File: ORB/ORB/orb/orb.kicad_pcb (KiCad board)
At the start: 2 copper layers, 132.1 x 82.5 mm, 6 parts, among them U1 Arduino_Nano, X1 14-Pin Plug, X2 14-Pin Plug, X3 14-Pin Plug, X4 14-Pin Plug

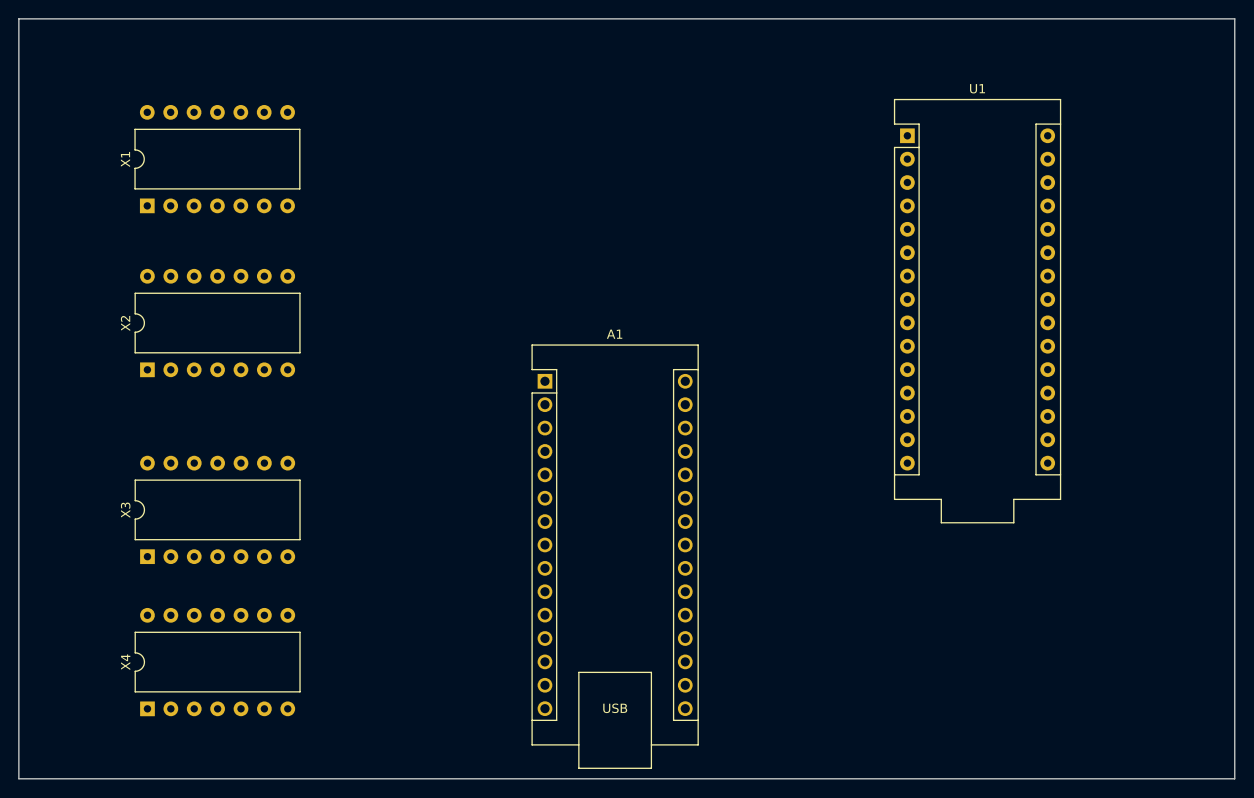
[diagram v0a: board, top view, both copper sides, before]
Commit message: Latest updates
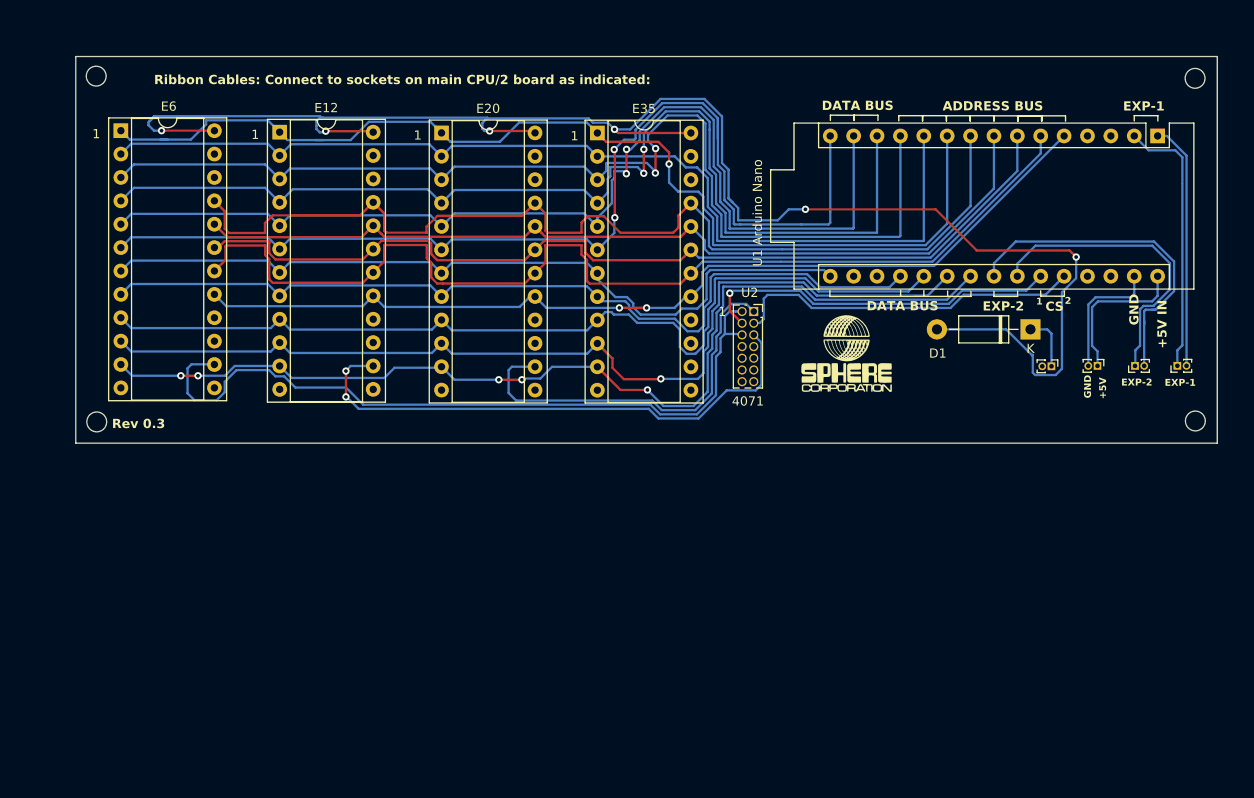
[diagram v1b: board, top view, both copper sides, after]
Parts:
- removed A1: Arduino_Nano_v3.x, Module:Arduino_Nano
- removed X1, X2, X3, X4: 14-Pin Plug, Package_DIP:DIP-14_W10.16mm
- added D1: 1N4001, Diode_THT:D_DO-41_SOD81_P10.16mm_Horizontal, F.Cu at (193.7, 75.6)
- added E12: MM1702A, Package_DIP:DIP-24_W10.16mm_Socket, F.Cu at (112.2, 54.2)
- added E20: MM1702A, Package_DIP:DIP-24_W10.16mm_Socket, F.Cu at (129.7, 54.3)
- added E35: MM1702A, Package_DIP:DIP-24_W10.16mm_Socket, F.Cu at (146.7, 54.3)
- added E6: MM1702A, Package_DIP:DIP-24_W10.16mm_Socket, F.Cu at (94.9, 54.1)
- added G***: LOGO, Arduino:sphere-corp-board-logo, F.Cu at (173.8, 78.2)
- added G***: LOGO, Arduino:orb-logo, B.Cu at (201.7, 61.2)
- added J1: Conn_01x02_Socket, Connector_PinHeader_1.00mm:PinHeader_1x02_P1.00mm_Vertical, F.Cu at (201.0, 79.6)
- added J2: Conn_01x02_Socket, Connector_PinHeader_1.00mm:PinHeader_1x02_P1.00mm_Vertical, F.Cu at (209.7, 79.6)
- added J3: Conn_01x02_Socket, Connector_PinHeader_1.00mm:PinHeader_1x02_P1.00mm_Vertical, F.Cu at (205.1, 79.6)
- added J4: Conn_01x02_Socket, Connector_PinHeader_1.00mm:PinHeader_1x02_P1.00mm_Vertical, F.Cu at (196.0, 79.7)
- added U3: 4071, Connector_PinSocket_1.27mm:PinSocket_2x07_P1.27mm_Vertical, F.Cu at (163.7, 73.7)
- moved U1 27.2 mm to (207.5, 54.6), turned to -90 degrees
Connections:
- U1 pad 1: unconnected-(U1-D1/TX-Pad1) -> Net-(J2-Pin_2)
- U1 pad 10: unconnected-(U1-D7-Pad10) -> Net-(E12-A2)
- U1 pad 11: unconnected-(U1-D8-Pad11) -> Net-(E12-A1)
- U1 pad 12: unconnected-(U1-~D9-Pad12) -> Net-(E12-A0)
- U1 pad 13: unconnected-(U1-~D10-Pad13) -> Net-(E12-D0)
- U1 pad 14: unconnected-(U1-~D11-Pad14) -> Net-(E12-D1)
- U1 pad 15: unconnected-(U1-D12-Pad15) -> Net-(E12-D2)
- U1 pad 16: unconnected-(U1-D13-Pad16) -> Net-(E12-D3)
- U1 pad 19: unconnected-(U1-A0/D14-Pad19) -> Net-(E12-D4)
- U1 pad 2: unconnected-(U1-D0/RX-Pad2) -> Net-(J2-Pin_1)
- U1 pad 20: unconnected-(U1-A1/D15-Pad20) -> Net-(E12-D5)
- U1 pad 21: unconnected-(U1-A2/D16-Pad21) -> Net-(E12-D6)
- U1 pad 22: unconnected-(U1-A3/D17-Pad22) -> Net-(E12-D7)
- U1 pad 23: unconnected-(U1-A4/D18-Pad23) -> Net-(J3-Pin_2)
- U1 pad 24: unconnected-(U1-A5/D19-Pad24) -> Net-(J3-Pin_1)
- U1 pad 25: unconnected-(U1-A6/D20-Pad25) -> Net-(U1-A6/D20)
- U1 pad 26: unconnected-(U1-A7/D21-Pad26) -> Net-(U1-A7/D21)
- U1 pad 29: unconnected-(U1-GND-Pad29) -> Net-(J1-Pin_2)
- U1 pad 30: unconnected-(U1-VIN-Pad30) -> Net-(J1-Pin_1)
- U1 pad 5: unconnected-(U1-D2-Pad5) -> Net-(E12-A7)
- U1 pad 6: unconnected-(U1-~D3-Pad6) -> Net-(E12-A6)
- U1 pad 7: unconnected-(U1-D4-Pad7) -> Net-(E12-A5)
- U1 pad 8: unconnected-(U1-~D5-Pad8) -> Net-(E12-A4)
- U1 pad 9: unconnected-(U1-~D6-Pad9) -> Net-(E12-A3)
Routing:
- net Net-(D1-A): track 0.00 -> 179.7 mm, vias 0 -> 6
- net Net-(E12-A0): track 0.00 -> 118.5 mm, vias 0 -> 2
- net Net-(E12-A2): track 0.00 -> 116.7 mm, vias 0 -> 1
- net Net-(E12-D0): track 0.00 -> 116.4 mm, vias 0 -> 2
- net Net-(E12-A6): track 0.00 -> 116.0 mm
- net Net-(E12-D2): track 0.00 -> 115.4 mm, vias 0 -> 2
- net Net-(E12-D1): track 0.00 -> 114.3 mm, vias 0 -> 2
- net Net-(E12-A3): track 0.00 -> 110.8 mm
- net Net-(E12-D7): track 0.00 -> 109.8 mm, vias 0 -> 5
- net Net-(E12-A1): track 0.00 -> 108.8 mm
- net Net-(E12-D6): track 0.00 -> 105.3 mm, vias 0 -> 1
- net Net-(E12-A7): track 0.00 -> 103.3 mm, vias 0 -> 2
- net Net-(E12-A5): track 0.00 -> 102.4 mm
- net Net-(E12-D5): track 0.00 -> 101.5 mm
- net Net-(E12-A4): track 0.00 -> 98.1 mm
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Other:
- board size 132.1 x 82.5 mm -> 124 x 42 mm
- board text added: "+5V"
- board text added: "+5V IN"
- board text added: "1"
- board text added: "2"
- board text added: "ADDRESS BUS"
- board text added: "CS"
- board text added: "DATA BUS"
- board text added: "EXP-1"
- board text added: "EXP-2"
- board text added: "GND"
- board text added: "Rev 0.3"
- board text added: "Ribbon Cables: Connect to sockets on main CPU/2 board as indicated:"
- board text added: "U1 Arduino Nano"
- board text added: "U2"
